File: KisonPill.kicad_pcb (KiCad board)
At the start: 4 copper layers, 44.7 x 46.8 mm, 47 parts, among them J1 USB_C_Receptacle_USB2.0, J2 Conn_01x17_Male, J3 Conn_01x17_Male, J4 Conn_01x03_Male, J5 Conn_01x04_Male, J6 Conn_01x03_Male, J7 Conn_01x08_Male, Q1 2N3904S-RTK/PS, Q2 2N3904S-RTK/PS, SW1 SW_Push, SW2 SW_Push, U1 CP2102N-A01-GQFN28, U2 ESP32-WROOM-32D, U3 SPX1117M3-L-3-3/TR, U4 ESP32FullConnector-KisonCommon, U5 ICM-20602, U6 USBLC6-2SC6-Power_Protection, U7 ESP32FullConnector

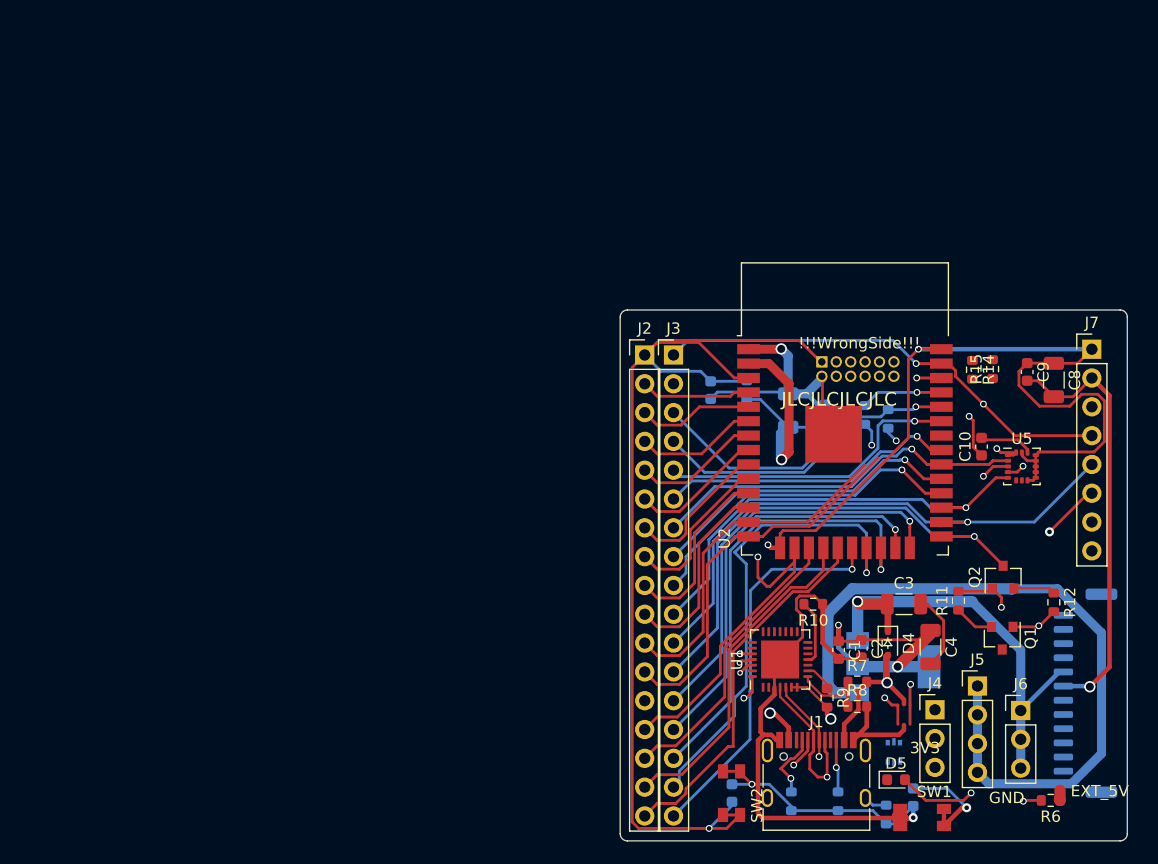
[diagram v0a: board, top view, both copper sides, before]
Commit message: V1
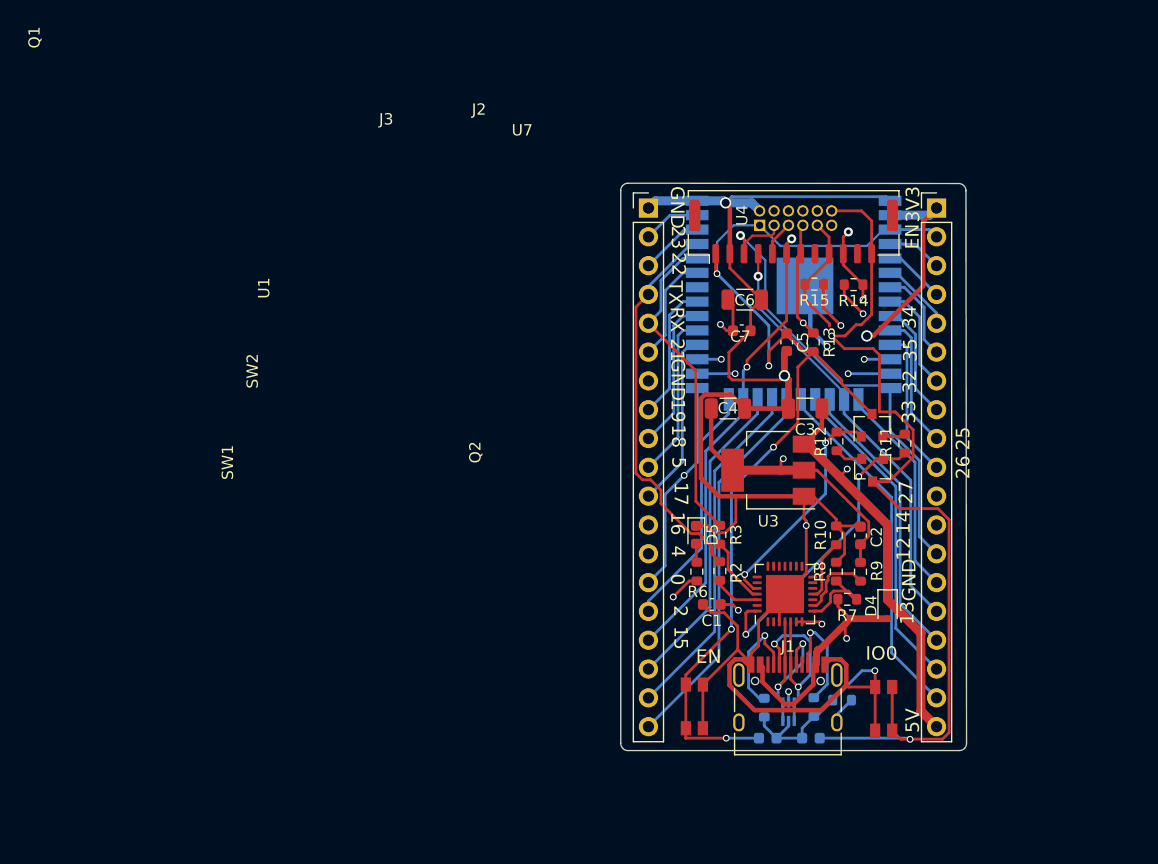
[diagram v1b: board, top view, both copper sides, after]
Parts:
- removed C10, C9: 0.1uf, Capacitor_SMD:C_0603_1608Metric
- removed C8: 10uf, Capacitor_SMD:C_1206_3216Metric
- removed J4, J6: Conn_01x03_Male, Connector_PinHeader_2.54mm:PinHeader_1x03_P2.54mm_Vertical
- removed J5: Conn_01x04_Male, Connector_PinHeader_2.54mm:PinHeader_1x04_P2.54mm_Vertical
- removed J7: Conn_01x08_Male, Connector_PinHeader_2.54mm:PinHeader_1x08_P2.54mm_Vertical
- removed U5: ICM-20602, Package_LGA:LGA-16_3x3mm_P0.5mm_LayoutBorder3x5y
- added G***: LOGO, KisonCommon:tamako100, B.Cu at (133.6, 96.8)
- C5, C6, C7, R13, R2, R3, U3, U4, U7: moved to F.Cu
- J2, J3: value Conn_01x17_Male -> Conn_01x19_Male; footprint Connector_PinHeader_2.54mm:PinHeader_1x17_P2.54mm_Vertical -> Connector_PinHeader_2.54mm:PinHeader_1x19_P2.54mm_Vertical
- U2: moved to B.Cu
- U6: footprint KisonCommon:USBLC6-2P6 -> KisonCommon:USBLC6-2P6-SOT666
- moved U7 48.1 mm to (134.4, 72.1), turned to 0 degrees
- moved R6 37.1 mm to (125.9, 102.1), turned to 90 degrees
- moved J2 28.8 mm to (147.0, 70.0)
- moved D5 27.9 mm to (125.8, 98.8), turned to 270 degrees
- moved C4 27.6 mm to (128.6, 87.7), turned to 0 degrees
- moved R12 23.8 mm to (138.2, 90.6), turned to 90 degrees
- moved Q1 22.0 mm to (141.3, 89.2), turned to 90 degrees
- moved U3 20.5 mm to (132.2, 93.1), turned to 180 degrees
- moved C3 19.3 mm to (135.4, 87.7), turned to 180 degrees
- moved R2 18.8 mm to (127.9, 102.0)
- moved R3 18.0 mm to (127.9, 98.8)
- moved R15 17.4 mm to (136.2, 76.7), turned to 180 degrees
- moved Q2 14.9 mm to (141.4, 93.1), turned to 270 degrees
- moved R11 14.6 mm to (144.2, 90.8), turned to 270 degrees
- moved U2 13.8 mm to (134.4, 77.6), turned to 180 degrees
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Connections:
- J2 pad 1: /EN -> +3V3
- J2 pad 10: /IO27 -> /IO26
- J2 pad 11: /IO14 -> /IO27
- J2 pad 12: /IO12 -> /IO14
- J2 pad 13: GND -> /IO12
- J2 pad 14: /IO13 -> GND
- J2 pad 15: /SD2 -> /IO13
- J2 pad 16: /SD3 -> /SD2
- J2 pad 17: /CMD -> /SD3
- J2 pad 2: /SENSOR_VP -> /EN
- J2 pad 3: /SENSOR_VN -> /SENSOR_VP
- J2 pad 4: /IO34 -> /SENSOR_VN
- J2 pad 5: /IO35 -> /IO34
- J2 pad 6: /IO32 -> /IO35
- J2 pad 7: /IO33 -> /IO32
- J2 pad 8: /IO25 -> /IO33
- J2 pad 9: /IO26 -> /IO25
- J3 pad 1: /IO23 -> GND
- J3 pad 10: /IO16 -> /IO5
- J3 pad 11: /IO4 -> /IO17
- J3 pad 12: /IO0 -> /IO16
- J3 pad 13: /IO2 -> /IO4
- J3 pad 14: /IO15 -> /IO0
- J3 pad 15: /SD1 -> /IO2
- J3 pad 16: /SD0 -> /IO15
- J3 pad 17: /CLK -> /SD1
- J3 pad 2: /IO22 -> /IO23
- J3 pad 3: /TXD0 -> /IO22
- J3 pad 4: /RXD0 -> /TXD0
- J3 pad 5: /IO21 -> /RXD0
- J3 pad 6: /IO19 -> /IO21
- J3 pad 7: /IO18 -> GND
- J3 pad 8: /IO5 -> /IO19
- J3 pad 9: /IO17 -> /IO18
- U4 pad 8: /EXT_5V -> Net-(U4-Pad8)
- U7 pad 10: /RXD0 -> Net-(R14-Pad1)
- U7 pad 8: /EXT_5V -> Net-(U7-Pad8)
- U7 pad 9: /TXD0 -> Net-(R15-Pad2)
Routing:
- net GND: track 314.3 -> 231.8 mm, vias 6 -> 5
- net /IO32: track 62.0 -> 9.41 mm, vias 1 -> 0
- net /IO0: track 72.4 -> 122.8 mm, vias 2 -> 3
- net +3V3: track 168.3 -> 118.6 mm
- net /IO35: track 56.0 -> 8.14 mm
- net /IO23: track 50.1 -> 5.09 mm, vias 3 -> 0
- net /IO18: track 52.9 -> 13.3 mm, vias 1 -> 0
- net /IO5: track 47.5 -> 14.6 mm, vias 1 -> 0
- net /EXT_5V: track 88.3 -> 57.3 mm, vias 1 -> 2
- net /TXD0: track 28.5 -> 56.9 mm
- net /IO4: track 50.3 -> 22.4 mm
- net /IO19: track 38.5 -> 12.0 mm, vias 2 -> 0
- net /TXD: track 29.2 -> 4.23 mm, vias 2 -> 0
- net /RXD0: track 27.1 -> 51.2 mm
- net /RXD: track 28.5 -> 6.00 mm, vias 2 -> 0
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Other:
- board size 44.7 x 46.8 mm -> 30.5 x 50 mm
- board text added: "0"
- board text added: "12"
- board text added: "13"
- board text added: "14"
- board text added: "15"
- board text added: "16"
- board text added: "17"
- board text added: "18"
- board text added: "19"
- board text added: "2"
- board text added: "21"
- board text added: "22"
- board text added: "23"
- board text added: "25"
- board text added: "26"
- board text added: "27"
- board text added: "32"
- board text added: "33"
- board text added: "34"
- board text added: "35"
- board text added: "4"
- board text added: "5"
- board text added: "5V"
- board text added: "EN"
- board text added: "IO0"
- board text added: "RX"
- board text added: "TX"
- board text removed: "EXT_5V"
